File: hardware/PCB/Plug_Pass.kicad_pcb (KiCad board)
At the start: 2 copper layers, 47.8 x 73.2 mm, 85 parts, among them IC1 DS3231M, IC2 PN532, IC3 VREG_SOT23-5, IC4 FT232RL, IC5 ATMEGA328P-AUR, J1 USB_B_Micro, J2 505568-0271, SW1 RESET, Y1 27.12MHz, Y2 16MHz

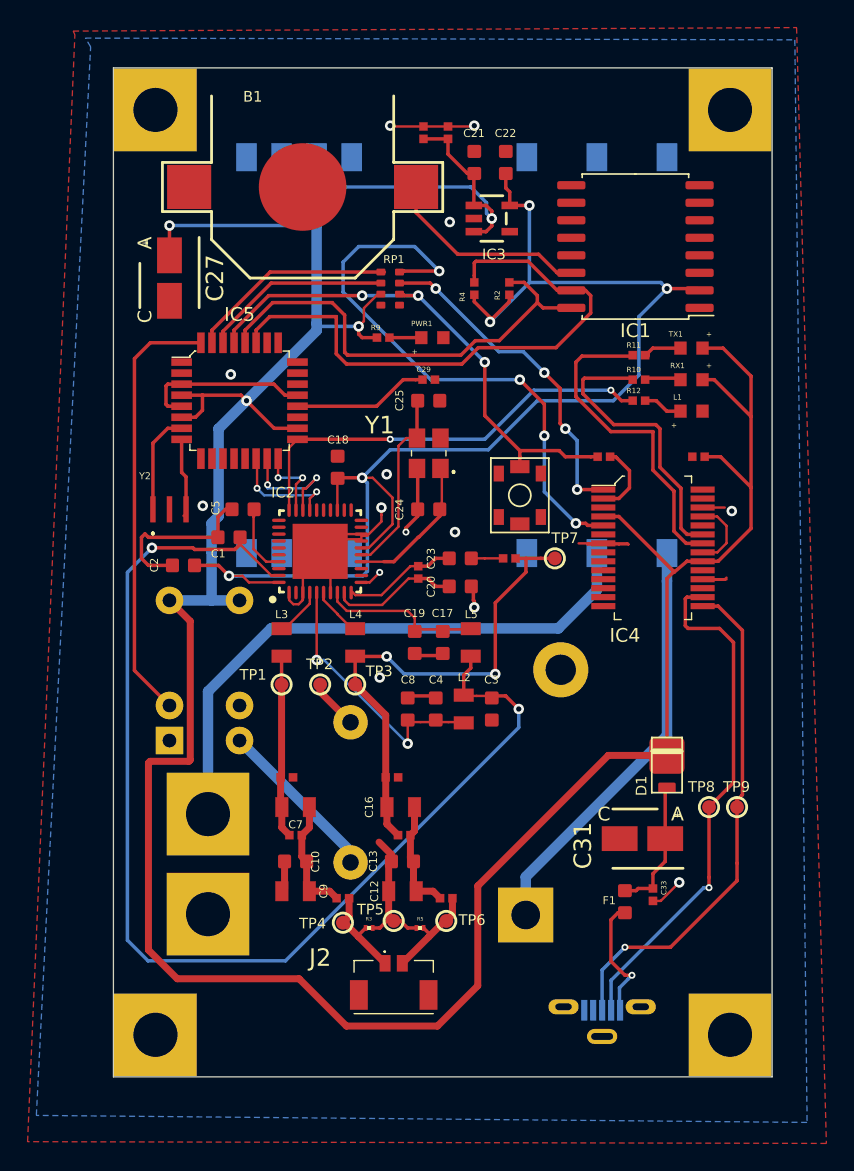
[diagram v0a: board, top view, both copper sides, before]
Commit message: Add files via upload
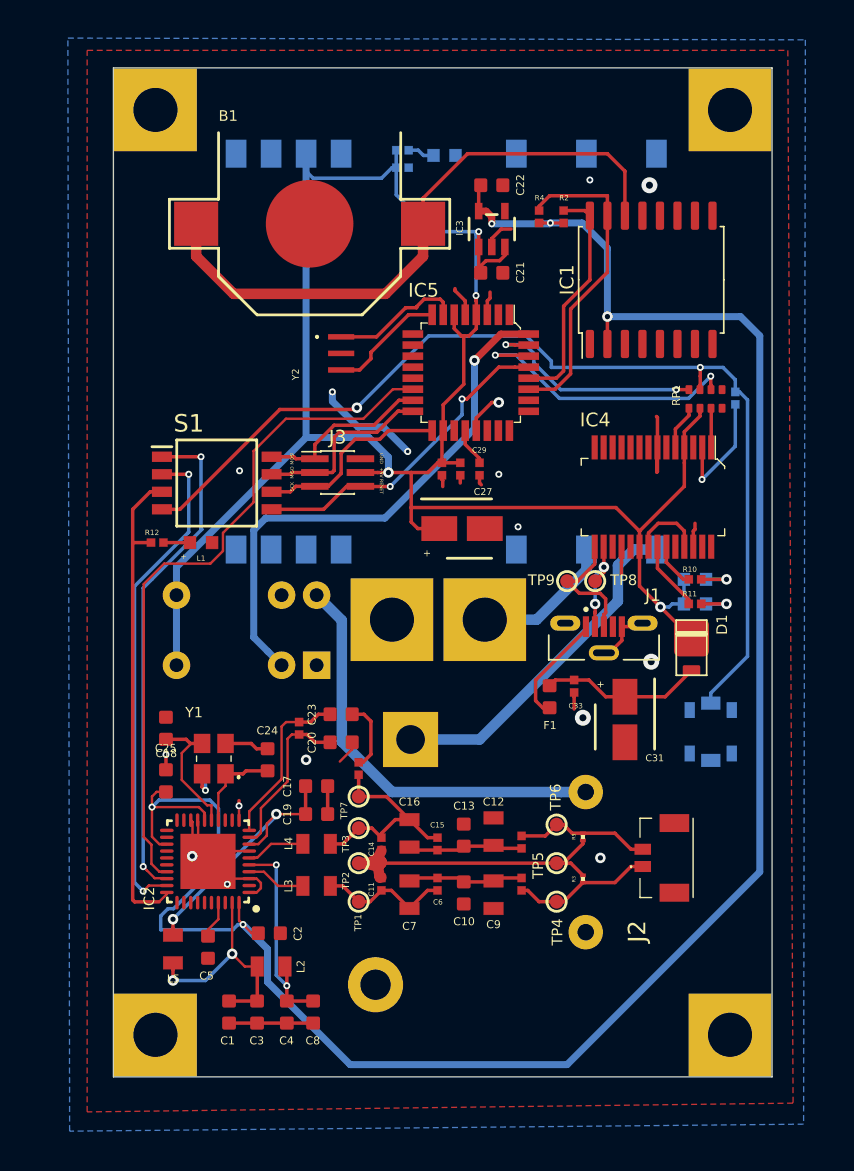
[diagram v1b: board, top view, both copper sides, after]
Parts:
- added J3: PinHeader_2x03_P1.00mm, Plug_Pass:PinHeader_2x03_P1.00mm_Vertical_SMD, F.Cu at (145.3, 82.7)
- added S1: 218-4LPST, Plug_Pass:SOIC127P844X265-8N, F.Cu at (136.5, 83.4)
- C30, C32, PWR1, R9, RX1, SW1, TX1: moved to B.Cu
- J1: moved to F.Cu
- moved RLY1 40.4 mm to (137.0, 98.7), turned to 270 degrees
- moved L1 36.8 mm to (135.4, 87.8)
- moved R12 36.4 mm to (132.2, 87.8)
- moved C1 34.4 mm to (137.4, 121.8), turned to 270 degrees
- moved C5 31.9 mm to (135.9, 117.1), turned to 270 degrees
- moved L5 31.0 mm to (133.3, 117.2)
- moved C25 30.4 mm to (132.8, 101.2), turned to 90 degrees
- moved C32 30.0 mm to (150.0, 60.6), turned to 0 degrees
- moved C27 27.9 mm to (154.3, 86.7), turned to 0 degrees
- moved J1 27.8 mm to (164.6, 93.6), turned to 0 degrees
- moved C3 27.8 mm to (139.4, 121.8)
- moved C2 27.4 mm to (140.3, 116.1), turned to 180 degrees
- moved Y1 27.1 mm to (136.3, 103.4)
- moved C18 25.9 mm to (132.8, 105.0)
- moved GND 25.2 mm to (149.2, 93.3)
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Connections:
- net Net-(C20-Pad2) renamed /VMID
- net Net-(C23-Pad2) renamed /RX1
- C30 pad 1: RESET -> RESET-1
- IC2 pad 28: MOSI -> MOSI-1
- IC2 pad 29: MISO -> MISO-1
- IC2 pad 30: SCK -> SCK-1
- R12 pad 1: SCK -> SCK-1
- RP1 pad 2: RESET -> Net-(IC5-Pad30)
- RP1 pad 3: RX -> RESET-1
- RP1 pad 4: TX -> Net-(IC5-Pad31)
- RP1 pad 5: Net-(IC5-Pad31) -> TX
- RP1 pad 6: Net-(IC5-Pad30) -> +5V
- RP1 pad 7: +5V -> RX
- SW1 pad 2: RESET -> RESET-1
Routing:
- net +5V: track 231.0 -> 147.8 mm
- net RESET-1: track 0.00 -> 75.1 mm, vias 0 -> 2
- net LDO: track 85.7 -> 16.8 mm
- net +3V3: track 96.6 -> 156.2 mm
- net SS: track 8.35 -> 50.2 mm, vias 2 -> 0
- net TX: track 42.6 -> 3.25 mm, vias 4 -> 0
- net MOSI-1: track 0.00 -> 36.4 mm, vias 0 -> 2
- net MISO-1: track 0.00 -> 35.9 mm, vias 0 -> 2
- net SCK-1: track 0.00 -> 35.2 mm
- net /NEUT: track 42.5 -> 10.3 mm
- net /D-: track 37.8 -> 7.35 mm, vias 1 -> 2
- net /BAT+: track 14.9 -> 45.0 mm
- net /D+: track 37.3 -> 9.16 mm, vias 1 -> 0
- net Net-(C14-Pad2): track 38.2 -> 15.7 mm, vias 2 -> 0
- net RX: track 24.3 -> 2.84 mm, vias 4 -> 0
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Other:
- board text added: "+5V"
- board text added: "Clatskanie People's Utility District Plug Pass - 120V Switch v3.1"
- board text added: "GND"
- board text added: "MISO"
- board text added: "MOSI"
- board text added: "RESET"
- board text added: "SCK"
- board text removed: "Clatskanie People's Utility District Plug Pass - 120V Switch v3.0"
